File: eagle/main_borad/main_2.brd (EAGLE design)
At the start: 50.8 x 45.7 mm, 35 parts, among them Q2 BSS123, Q3 BSS123, Q5 BSS123, Q6 BSS123, U1 XMEGA-A4TQFP

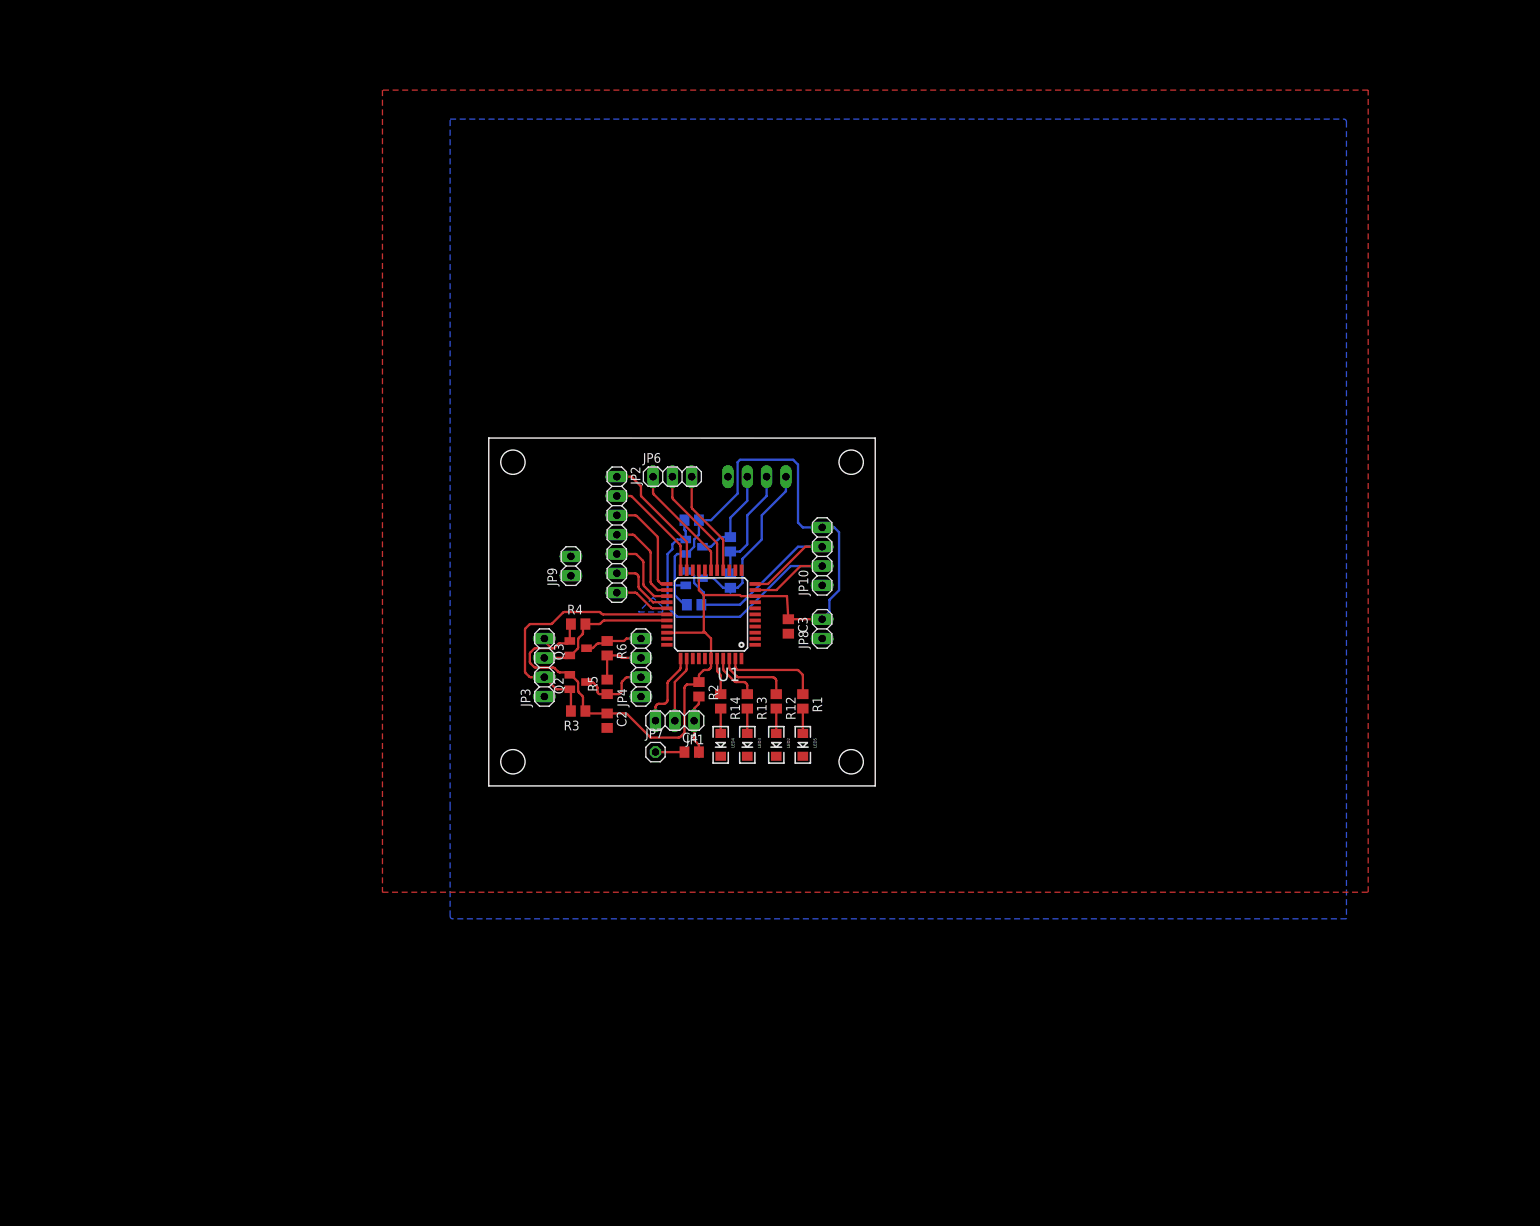
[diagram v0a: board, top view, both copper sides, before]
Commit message: main_board, ver 3.0
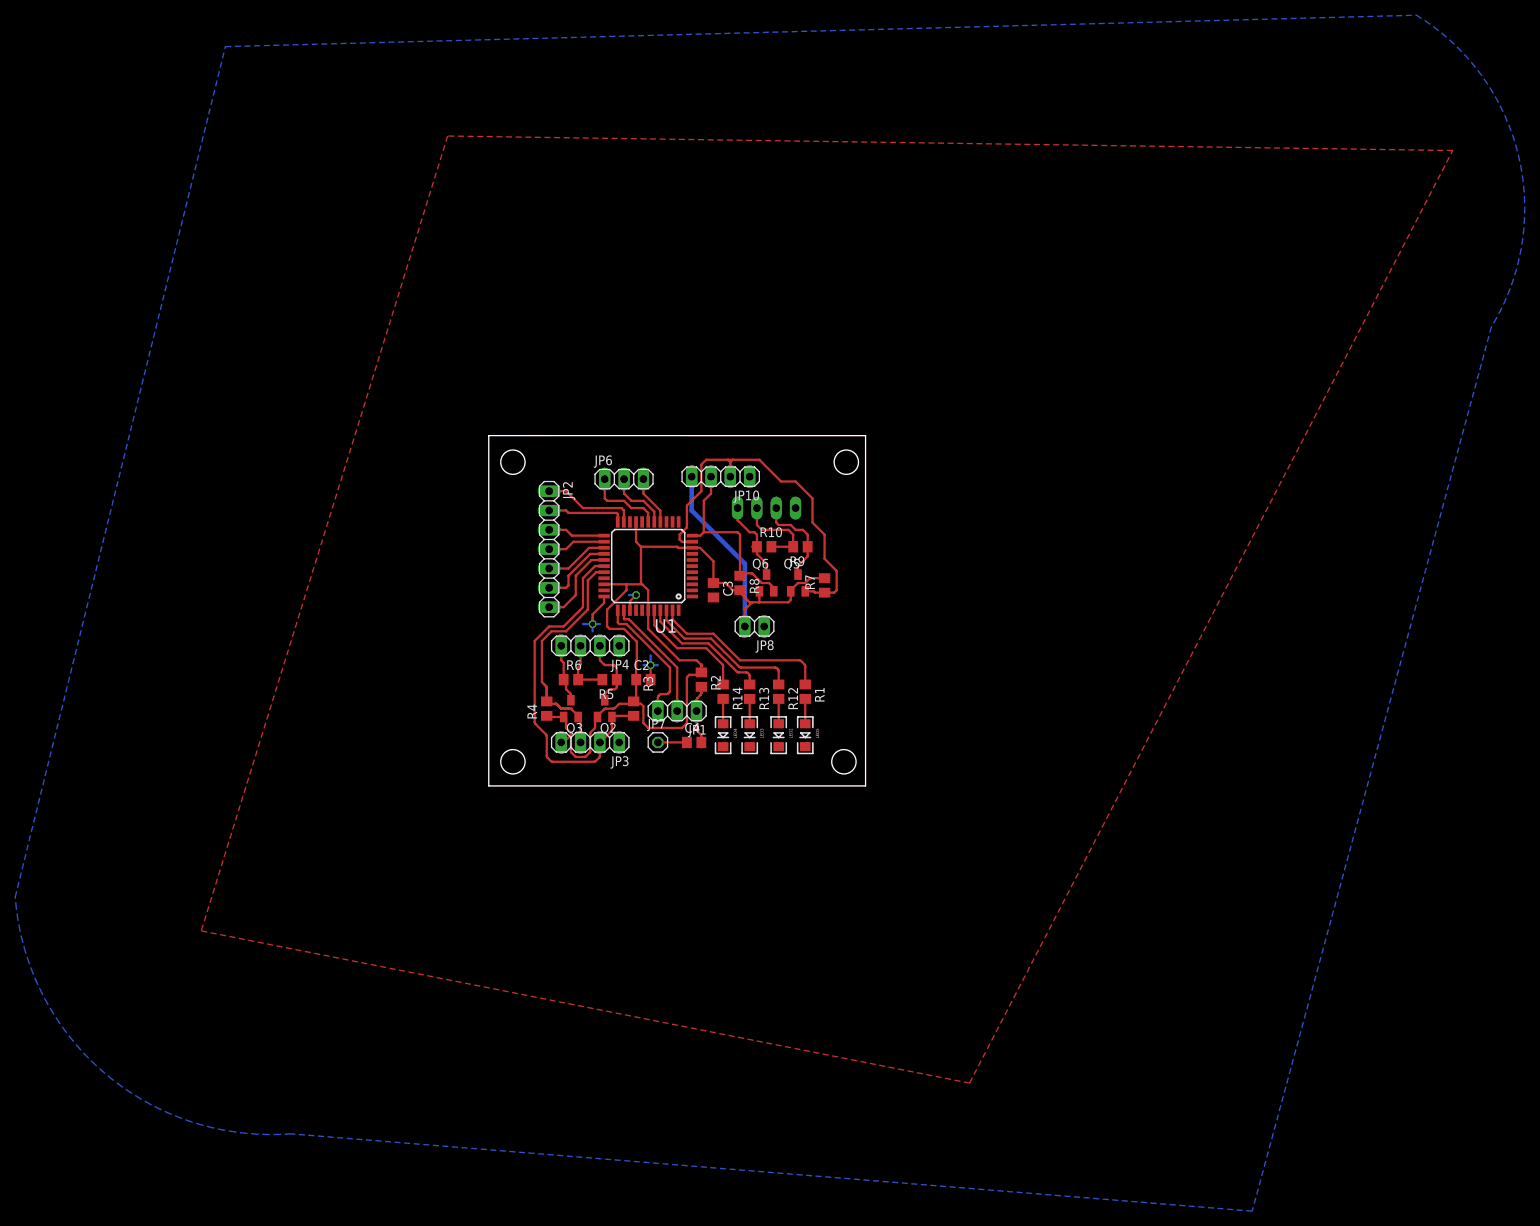
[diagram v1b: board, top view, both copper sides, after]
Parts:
- removed JP9: (no value), pinhead:1X02
- moved R7 19.5 mm to (44.1, 26.4), flipped to the top, turned to 90 degrees
- moved JP10 17.0 mm to (30.5, 40.6), turned to 180 degrees
- moved Q5 14.5 mm to (40.6, 26.7), flipped to the top, turned to 0 degrees
- moved R4 11.9 mm to (7.62, 10.2), turned to 270 degrees
- moved JP3 11.5 mm to (13.3, 5.71), turned to 180 degrees
- moved C3 10.9 mm to (29.5, 25.7)
- moved U1 10.4 mm to (21.0, 28.9)
- moved Q6 9.55 mm to (36.5, 26.7), flipped to the top, turned to 0 degrees
- moved R9 9.21 mm to (41.0, 31.4), flipped to the top, turned to 180 degrees
- moved JP2 9.09 mm to (7.94, 31.1)
- moved JP8 8.90 mm to (34.9, 21.0), turned to 180 degrees
- moved Q3 7.99 mm to (10.8, 10.2), turned to 0 degrees
- moved R3 7.31 mm to (19.1, 10.2), turned to 90 degrees
- moved JP4 7.25 mm to (13.3, 18.4), turned to 180 degrees
- moved C2 7.20 mm to (20.3, 14.0), turned to 0 degrees
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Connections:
- net GND: no longer JP9.1
- net VCC: no longer JP9.2
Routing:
- net GND: track 0.00 -> 16.7 mm, vias 0 -> 3
- net SCL1: track 20.0 -> 36.7 mm
- net SDA1: track 35.0 -> 47.5 mm
- net N$19: track 23.0 -> 11.3 mm
- net N$24: track 4.83 -> 15.7 mm
- net N$23: track 6.65 -> 17.4 mm
- net N$22: track 9.95 -> 20.6 mm
- net N$21: track 13.0 -> 23.6 mm
- net SCL0: track 35.6 -> 25.4 mm
- net N$11: track 9.98 -> 17.8 mm
- net N$2: track 8.80 -> 16.5 mm
- net N$17: track 14.0 -> 6.56 mm
- net N$16: track 14.7 -> 8.21 mm
- net N$7: track 13.6 -> 7.53 mm
- net N$4: track 15.4 -> 10.2 mm
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- removed copper zone on layer 16, net N$3
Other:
- board size 50.8 x 45.7 mm -> 49.5 x 46 mm

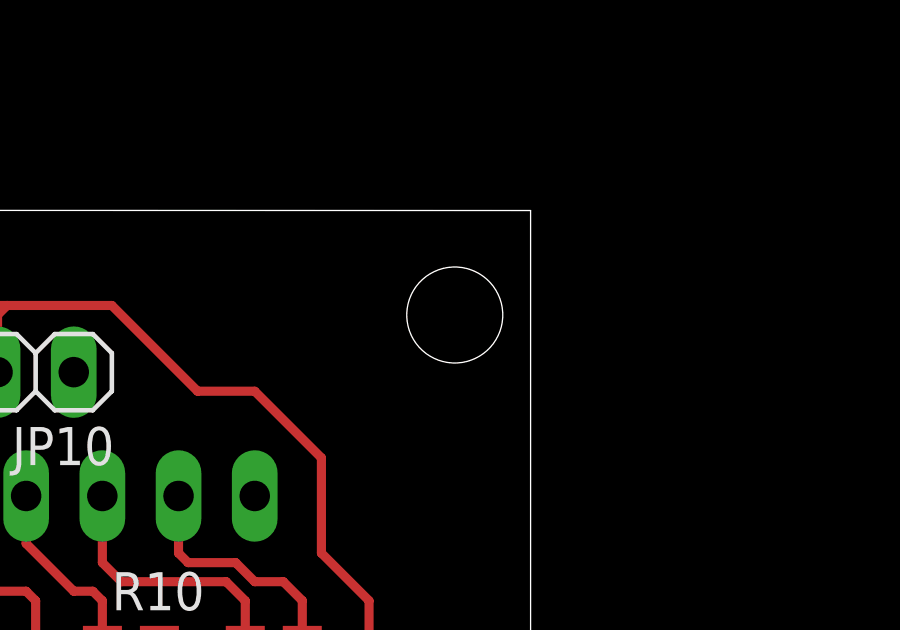
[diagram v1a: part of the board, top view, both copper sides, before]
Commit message: PCB ver. 4.0
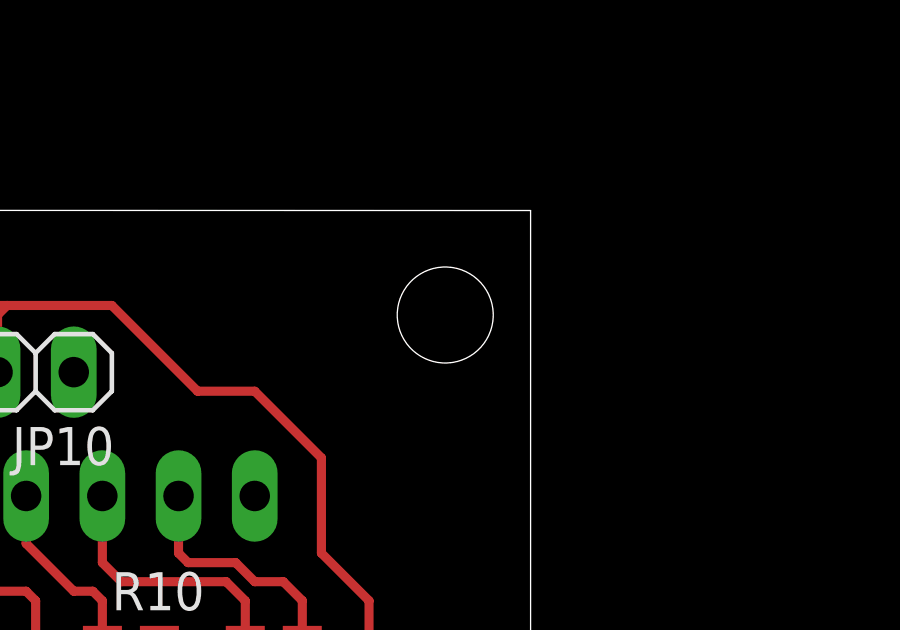
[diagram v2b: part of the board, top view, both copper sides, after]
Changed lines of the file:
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@@
 <wire x1="0" y1="46.0375" x2="0" y2="0" width="0" layer="20"/>
 <hole x="3.175" y="42.545" drill="3.2"/>
-<hole x="46.99" y="42.545" drill="3.2"/>
+<hole x="46.6725" y="42.545" drill="3.2"/>
 <hole x="46.6725" y="3.175" drill="3.2"/>
 <hole x="3.175" y="3.175" drill="3.2"/>

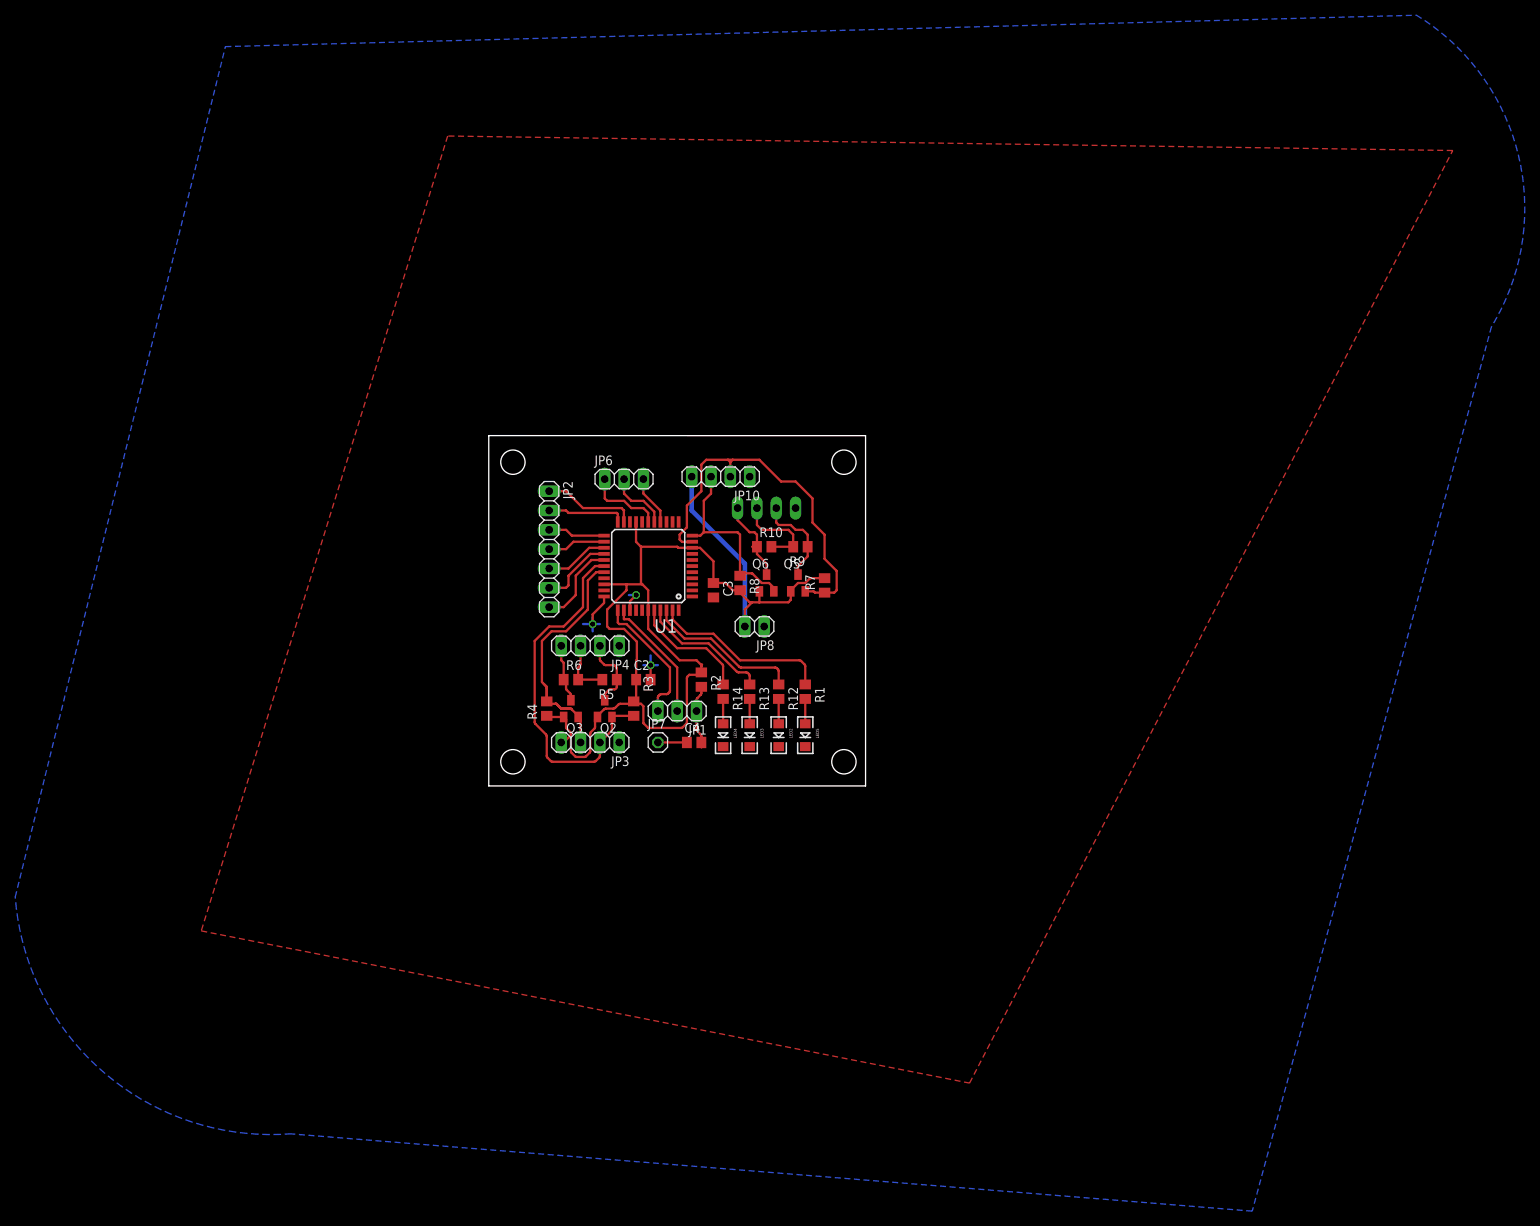
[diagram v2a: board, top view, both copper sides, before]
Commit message: PCB layout 6.0
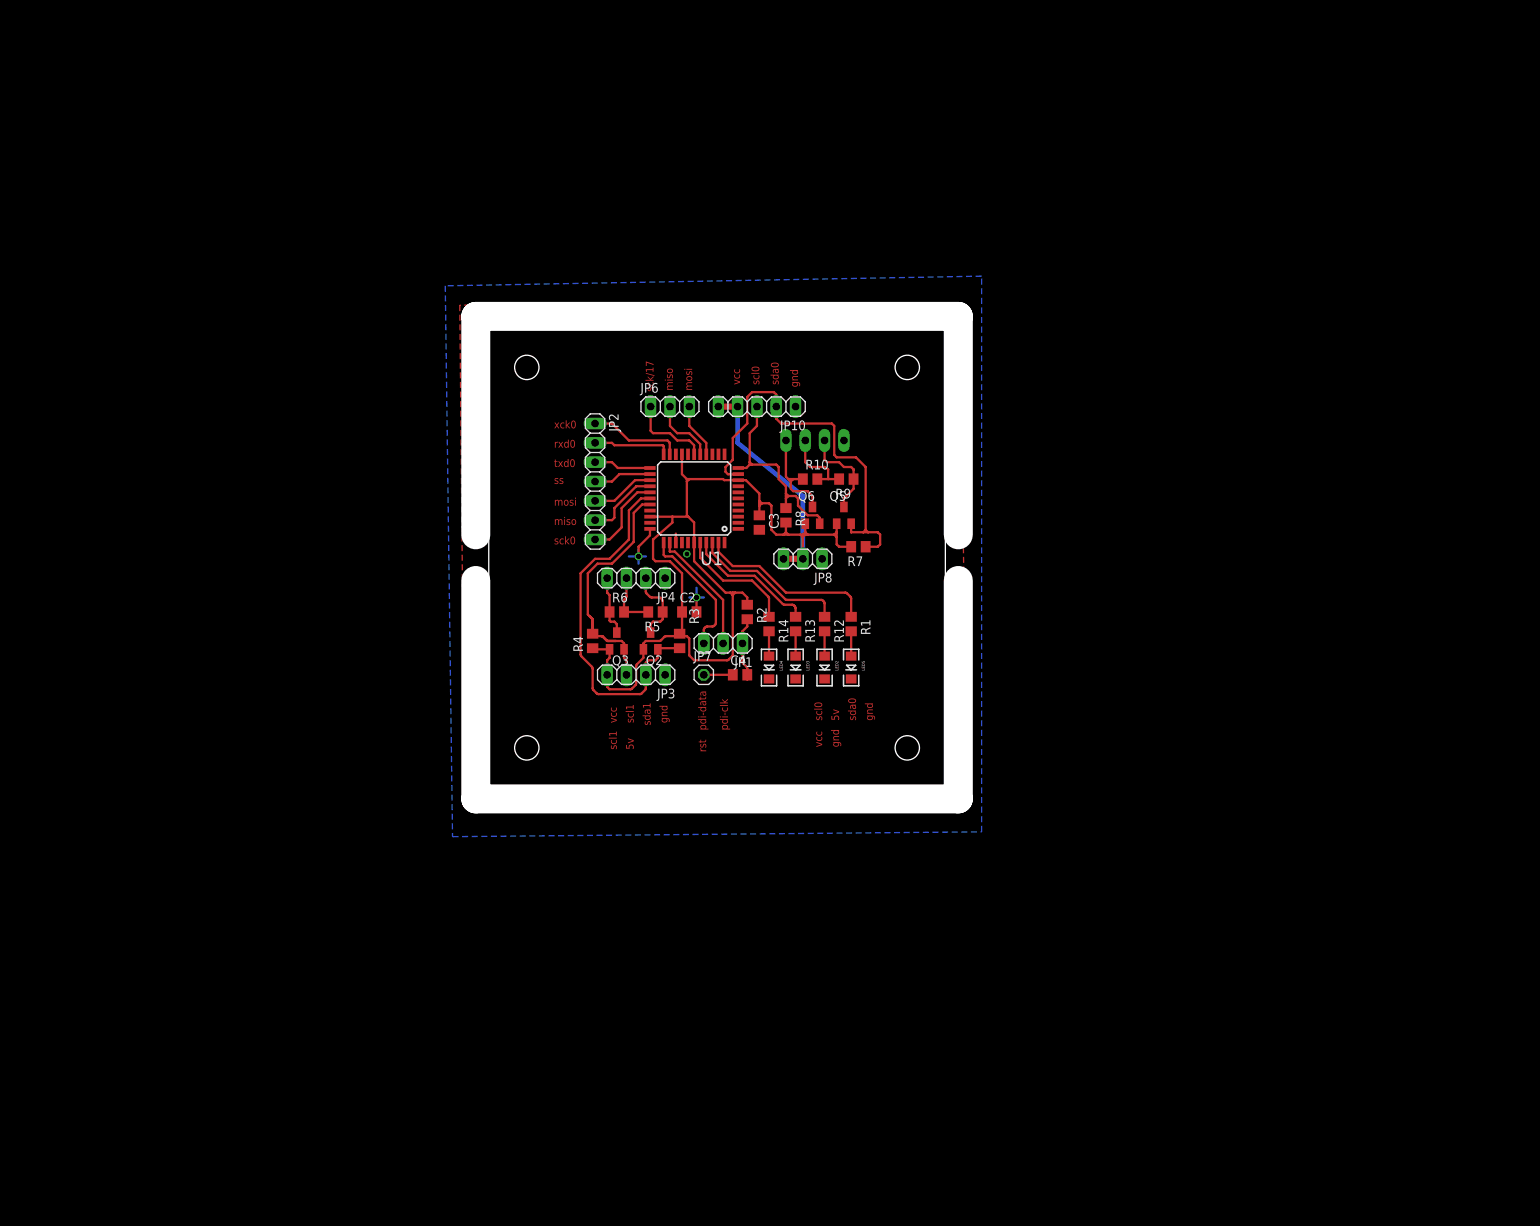
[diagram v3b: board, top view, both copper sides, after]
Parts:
- JP10: device pinhead:1X04 -> pinhead:1X05
- JP8: device pinhead:1X02 -> pinhead:1X03
- moved JP6 11.3 mm to (23.8, 49.8)
- moved JP8 10.9 mm to (41.3, 29.8)
- moved JP5 10.9 mm to (42.9, 45.4)
- moved JP2 10.7 mm to (14.0, 40.0)
- moved C3 10.7 mm to (35.6, 34.6)
- moved C4 10.7 mm to (33.0, 14.6)
- moved JP1 10.7 mm to (30.8, 18.7)
- moved Q2 10.7 mm to (21.3, 19.1)
- moved Q3 10.7 mm to (16.8, 19.1)
- moved R4 10.7 mm to (13.7, 19.1)
- moved U1 10.7 mm to (27.0, 37.8)
- moved C2 10.7 mm to (26.4, 22.9)
- moved JP3 10.7 mm to (19.4, 14.6)
- moved JP4 10.7 mm to (19.4, 27.3)
- moved JP7 10.7 mm to (28.3, 14.6)
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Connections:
- net VCC: now also JP10.5, JP8.3
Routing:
- net VCC: track 150.3 -> 165.4 mm
- net SDA0: track 50.3 -> 54.4 mm
- net SCL0: track 25.4 -> 28.2 mm
- net N$19: track 11.3 -> 14.0 mm
- net GND: track 16.7 -> 14.6 mm, vias 3 -> 5
- net N$20: track 12.0 -> 10.4 mm
- net SCL1: track 36.7 -> 37.4 mm
- net N$16: track 8.21 -> 8.84 mm
- net N$4: track 10.2 -> 10.9 mm
- net N$17: track 6.56 -> 7.19 mm
- net SDA1: track 47.5 -> 48.1 mm
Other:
- board size 49.5 x 46 mm -> 63.4 x 63.4 mm
- board text added: "5v"
- board text added: "gnd"
- board text added: "miso"
- board text added: "mosi"
- board text added: "pdi-clk"
- board text added: "pdi-data"
- board text added: "rst"
- board text added: "rxd0"
- board text added: "sck/17"
- board text added: "sck0"
- board text added: "scl0"
- board text added: "scl1"
- board text added: "sda0"
- board text added: "sda1"
- board text added: "ss"
- board text added: "txd0"
- board text added: "vcc"
- board text added: "xck0"
